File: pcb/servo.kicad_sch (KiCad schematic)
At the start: 1 part, among them J24 Conn_01x03_Pin

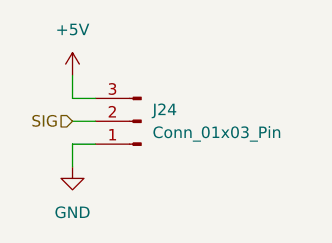
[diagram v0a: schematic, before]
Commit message: Add power switch
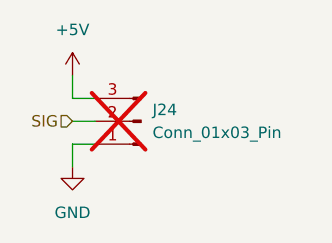
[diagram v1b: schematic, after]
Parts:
- J24: now not fitted
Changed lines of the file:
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@@
 		(in_bom yes)
 		(on_board yes)
-		(dnp no)
+		(dnp yes)
 		(property "Reference" "J24"
 			(at 90.17 59.6899 0)
